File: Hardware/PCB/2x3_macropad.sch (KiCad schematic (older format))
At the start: 18 parts, among them K1 KEYSW, K2 KEYSW, K3 KEYSW, K4 KEYSW, K5 KEYSW, K6 KEYSW, SW1 SW_PUSH, SW2 Rotary_Encoder_Switch, SW3 Rotary_Encoder_Switch, U1 ProMicro

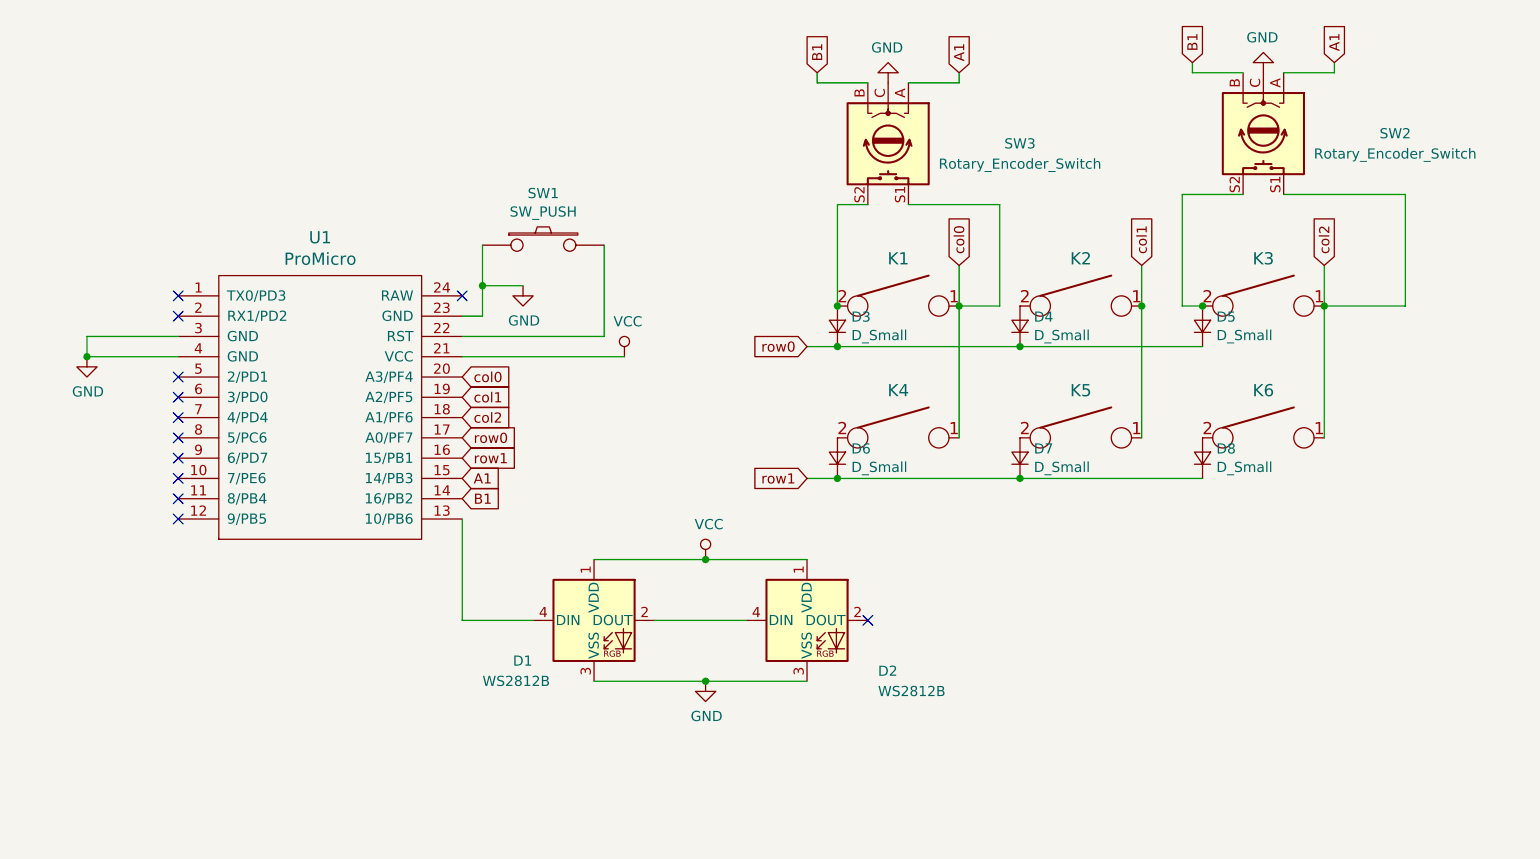
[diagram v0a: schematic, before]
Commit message: schematic fixes
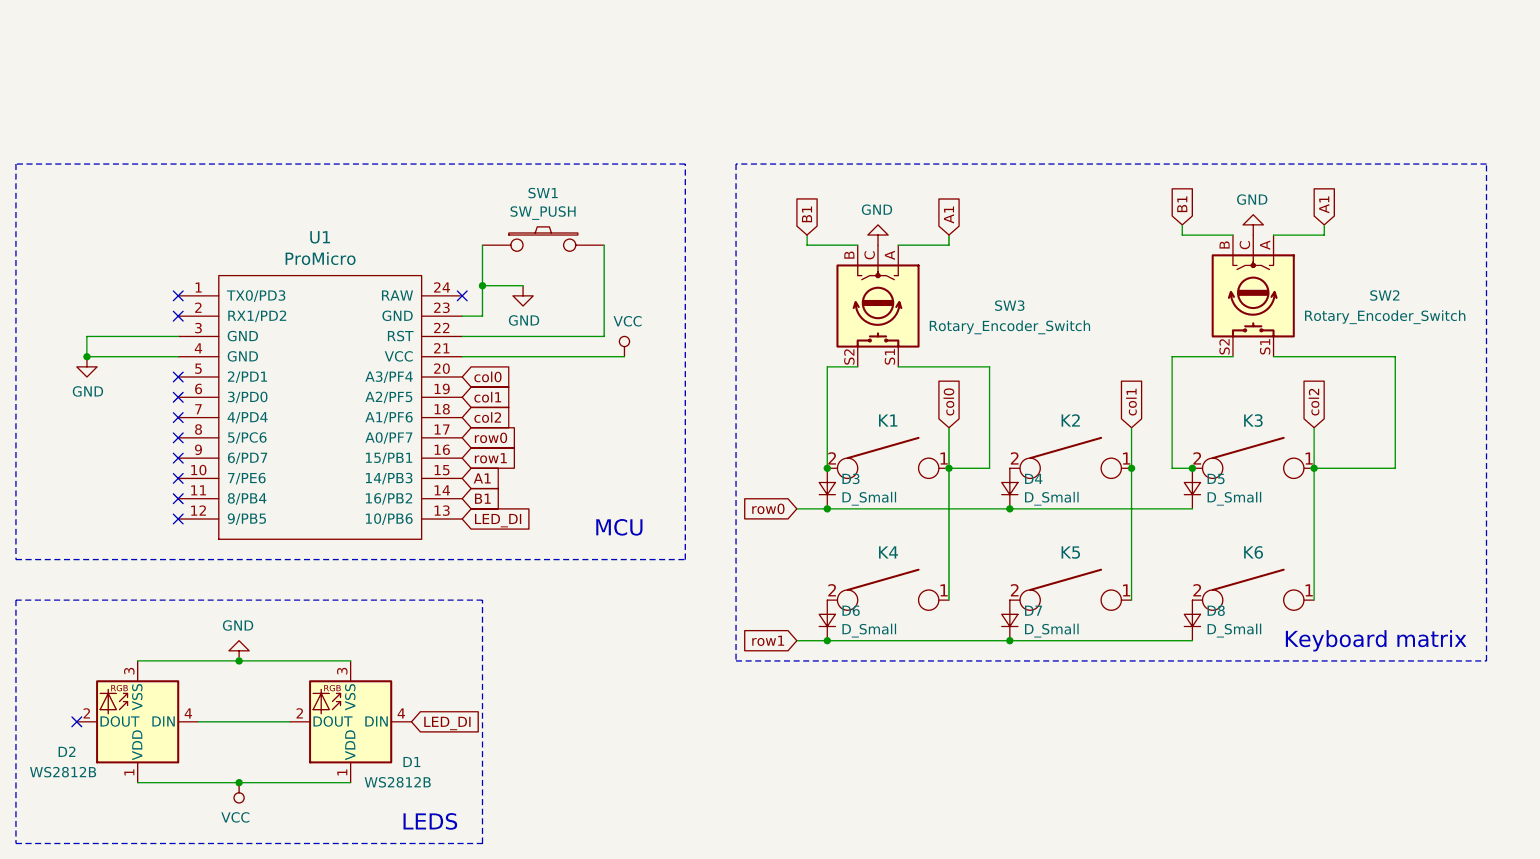
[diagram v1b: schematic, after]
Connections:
- net LED_DI: now reaches D1.4 (DIN), U1.13 (10/PB6)
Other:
- note added: "Keyboard matrix"
- note added: "LEDS"
- note added: "MCU\n"
- moved on the sheet: D1, D2, D3, D4, D5, D6, D7, D8, K1, K2, K3, K4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
